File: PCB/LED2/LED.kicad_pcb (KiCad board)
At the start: 2 copper layers, 70 x 70 mm, 29 parts, among them J1 Conn_01x03, J2 USB-C, U1 ESP32-PICO-MINI-02, U2 QR, U3 MD8942, U4 Barcode, U5 CH340X

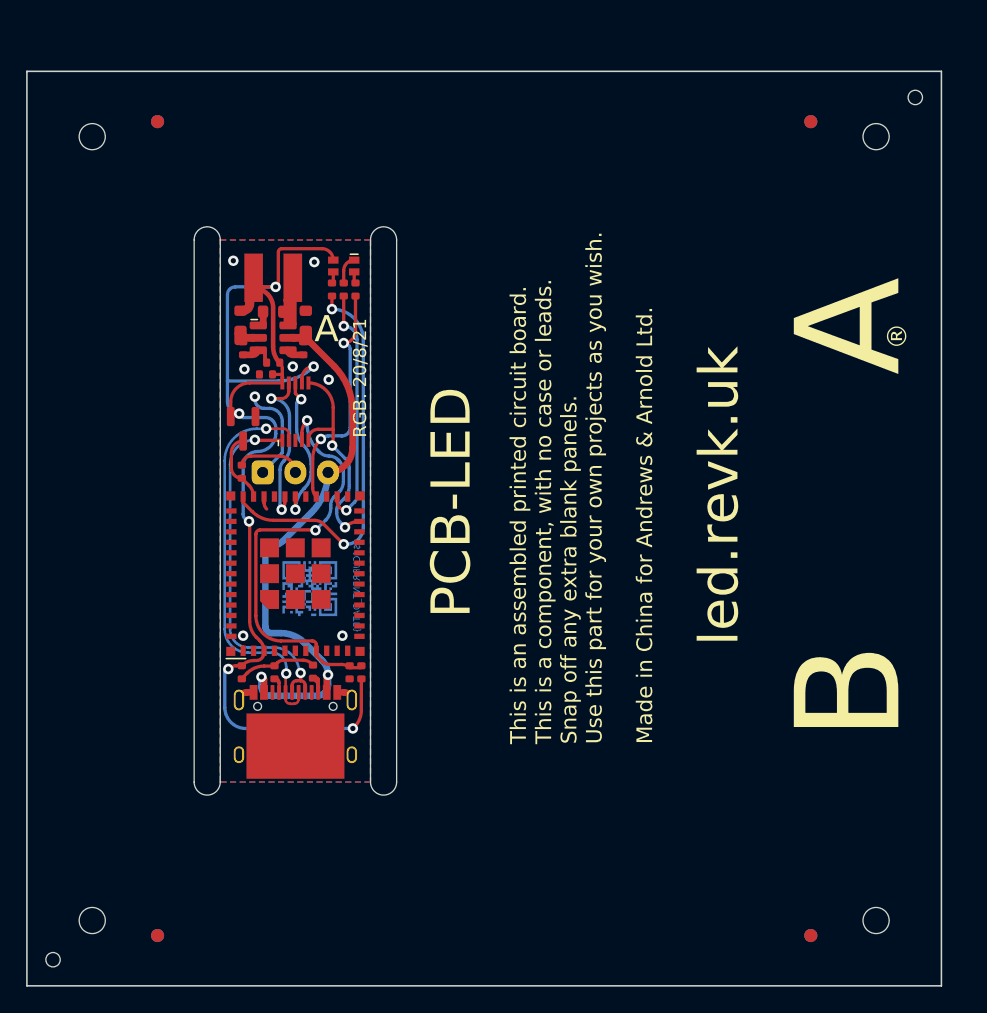
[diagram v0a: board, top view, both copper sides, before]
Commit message: Started tracking
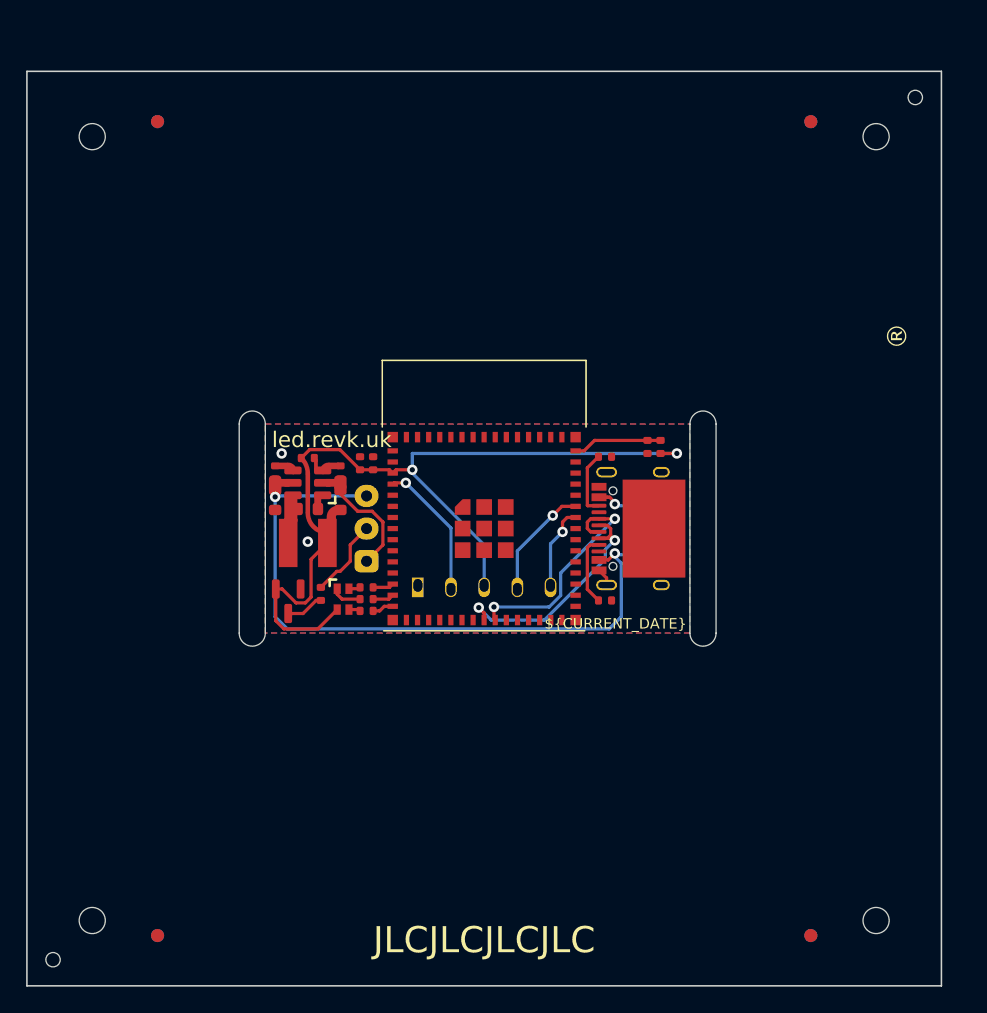
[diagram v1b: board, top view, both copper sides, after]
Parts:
- removed C1: 1uF, RevK:C_0402
- removed C2: 10uF 50V, RevK:C_0603_
- removed C3: 10uF 6.3V, RevK:C_0603_
- removed C4: 100nF, RevK:C_0603_
- removed C5, C6: 100nF, RevK:C_0402
- removed L1: 10uH, RevK:L_4x4_
- removed R1: 10k, RevK:R_0402
- removed R10: 40k2, RevK:R_0402_
- removed R13: 1M, RevK:R_0402_
- removed R9: 124k, RevK:R_0402_
- removed U1: ESP32-PICO-MINI-02, RevK:ESP32-PICO-MINI-02
- removed U2: QR, RevK:QR-LED
- removed U3: MD8942, RevK:SOT-23-6-MD8942
- removed U5: CH340X, RevK:CH340X
- added C10: 10uF 50V, RevK:C_0603_, F.Cu at (84.0, 97.8)
- added C11: 10uF 6.3V, RevK:C_0603_, F.Cu at (89.0, 97.8)
- added C12: 100nF, RevK:C_0603_, F.Cu at (86.5, 98.5)
- added C7: 100nF, RevK:C_0402, F.Cu at (91.5, 95.0)
- added C8: 22uF, RevK:C_0402, F.Cu at (90.5, 95.0)
- added C9: 1uF, RevK:C_0402, F.Cu at (112.5, 93.8)
- added J3: Shelly, RevK:Shelly, B.Cu at (100.0, 104.5)
- added L2: 10uH, RevK:L_4x4_, F.Cu at (86.5, 101.1)
- added R14: 39k2, RevK:R_0402_, F.Cu at (89.0, 95.7)
- added R15: 1M, RevK:R_0402_, F.Cu at (84.0, 95.7)
- added R2: 10K, RevK:R_0402, F.Cu at (113.5, 93.8)
- added R4: 124k, RevK:R_0402_, F.Cu at (86.5, 94.6)
- added U6: ESP32-S3-MINI-1, RevK:ESP32-S3-MINI-1, F.Cu at (100.0, 100.0)
- added U7: MD8942, RevK:SOT-23-6-MD8942, F.Cu at (86.5, 96.5)
- moved U4 31.3 mm to (118.5, 108.4), turned to 180 degrees
- moved J2 29.8 mm to (111.2, 100.0), turned to 90 degrees
- moved R6 27.8 mm to (109.2, 94.5), turned to 180 degrees
- moved R5 25.9 mm to (109.2, 105.5), turned to 0 degrees
- moved D2 25.5 mm to (89.2, 105.4), turned to -90 degrees
- moved R12 24.7 mm to (91.0, 106.3), turned to 0 degrees
- moved R8 23.8 mm to (91.0, 105.4), turned to 0 degrees
- moved R11 22.8 mm to (91.0, 104.5), turned to 0 degrees
- moved V1 14.1 mm to (100.0, 92.0)
- moved D3 13.6 mm to (85.0, 105.6)
- moved V2 11.4 mm to (100.0, 108.0)
- moved R7 11.1 mm to (87.5, 105.0)
- moved J1 6.94 mm to (91.0, 100.0), turned to 90 degrees
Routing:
- net EN: track 33.5 -> 0.00 mm, vias 2 -> 0
- net B: track 30.5 -> 1.64 mm, vias 2 -> 0
- net +3V3: track 83.6 -> 59.5 mm, vias 6 -> 2
- net R: track 18.7 -> 1.62 mm, vias 2 -> 0
- net GPIO0: track 16.7 -> 0.00 mm, vias 2 -> 0
- net G: track 18.1 -> 1.60 mm, vias 2 -> 0
- net DC: track 43.1 -> 58.5 mm, vias 2 -> 3
- net O: track 12.8 -> 0.00 mm, vias 2 -> 0
- net D-: track 30.4 -> 18.6 mm
- net I: track 11.7 -> 0.00 mm, vias 2 -> 0
- net Net-(J3-0): track 0.00 -> 10.6 mm, vias 0 -> 1
- net D+: track 27.9 -> 17.8 mm
- net Net-(J3-Rx): track 0.00 -> 8.81 mm, vias 0 -> 1
- net GND: track 17.4 -> 9.35 mm, vias 8 -> 2
- net Net-(U6-EN): track 0.00 -> 6.83 mm
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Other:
- board text added: "5060634238090"
- board text added: "Made in China for Andresw&Arnold Ltd"
- board text removed: "${TITLE}"
- board text removed: "22"
- board text removed: "RGB: 20/8/21"
- board text removed: "This is an assembled printed circuit board. This is a component, with no case or leads. Snap off any extra blank panels. Use this part for your own projects as you wish. Made in China for Andrews & Arnold Ltd."

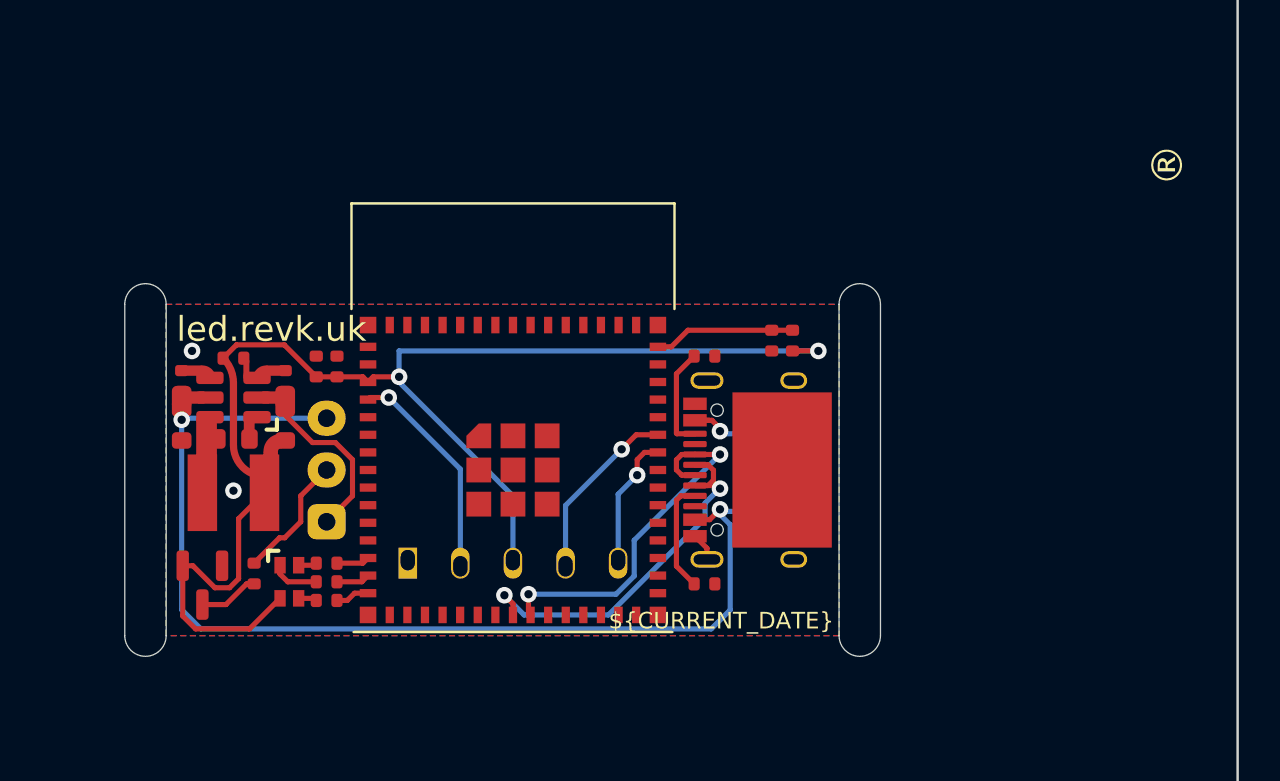
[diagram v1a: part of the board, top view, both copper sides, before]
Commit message: Tracked
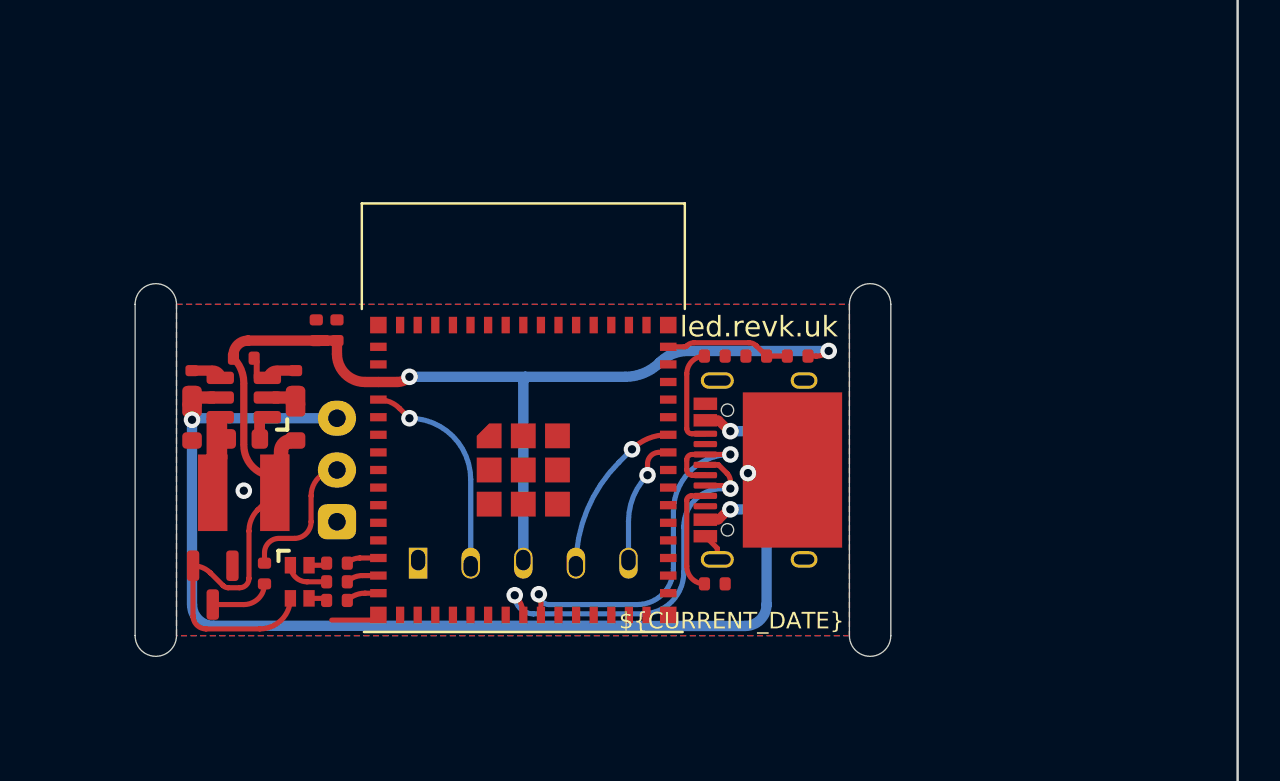
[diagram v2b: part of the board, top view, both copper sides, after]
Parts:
- moved C7 1.75 mm to (91.5, 93.2)
- moved C8 1.75 mm to (90.5, 93.2)
- moved C9 1.06 mm to (111.8, 94.5), turned to 180 degrees
- moved R2 0.79 mm to (113.8, 94.5), turned to 180 degrees
- moved C10 0.50 mm to (84.5, 97.8)
- moved C11 0.50 mm to (89.5, 97.8)
- moved C12 0.50 mm to (87.0, 98.5)
- moved D2 0.50 mm to (89.7, 105.4)
- moved D3 0.50 mm to (85.5, 105.6)
- moved J1 0.50 mm to (91.5, 100.0)
- moved J2 0.50 mm to (111.8, 100.0)
- moved J3 0.50 mm to (100.5, 104.5)
- moved L2 0.50 mm to (87.0, 101.1)
- moved R11 0.50 mm to (91.5, 104.5)
- moved R12 0.50 mm to (91.5, 106.3)
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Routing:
- net GND: track 9.35 -> 3.61 mm
- net DC: track 58.5 -> 61.0 mm
- net +3V3: track 59.5 -> 57.6 mm
- net D+: track 17.8 -> 19.4 mm
- net D-: track 18.6 -> 19.5 mm
- net Net-(U6-EN): track 6.83 -> 6.04 mm
- net Net-(J1-Pin_2): track 6.10 -> 6.71 mm
- net Net-(J3-Rx): track 8.81 -> 8.30 mm
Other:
- board text removed: "®"

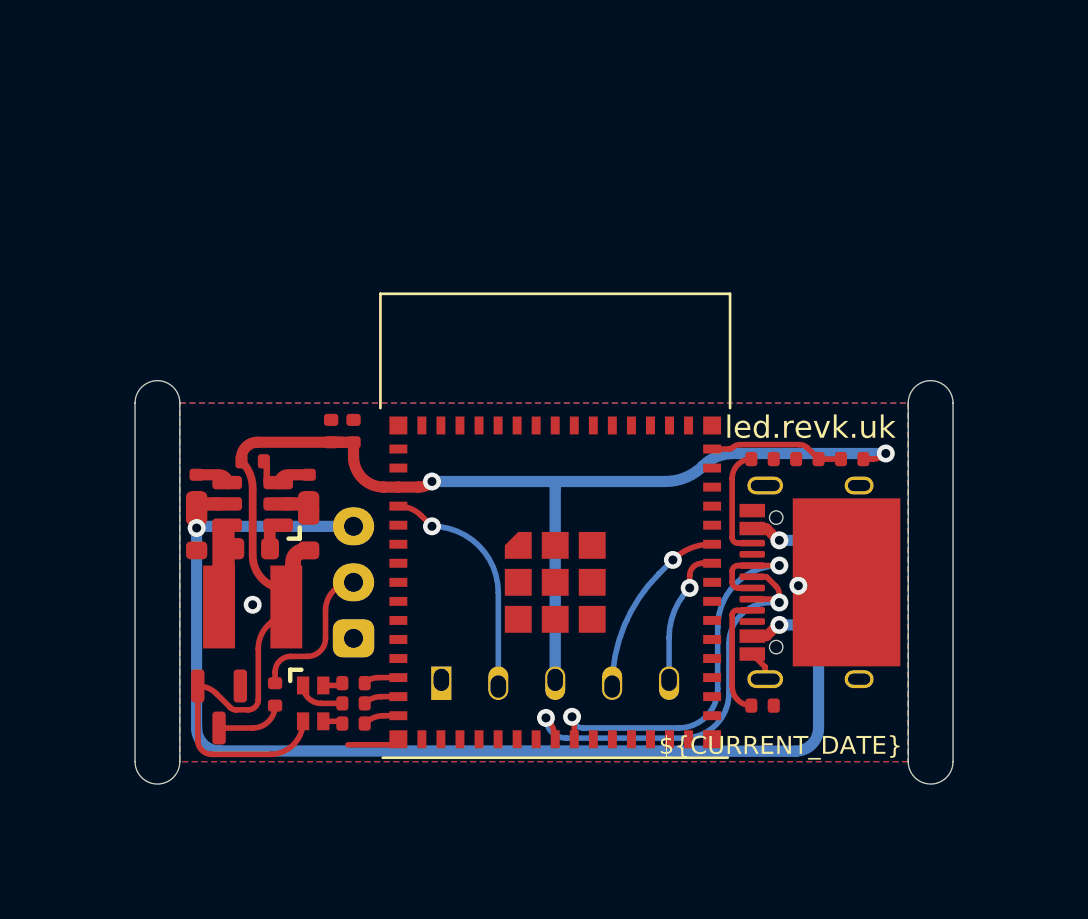
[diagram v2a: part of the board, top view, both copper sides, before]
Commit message: New S3
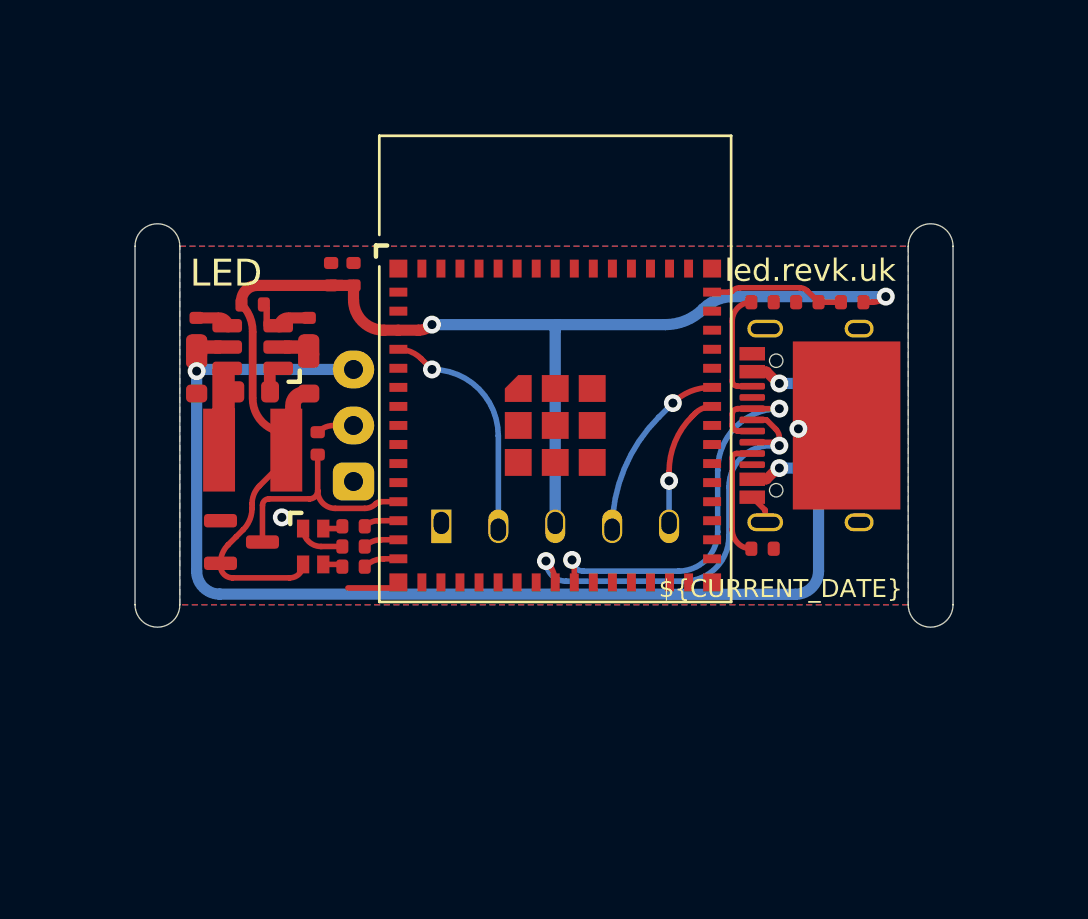
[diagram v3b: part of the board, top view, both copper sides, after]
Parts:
- moved R7 11.4 mm to (89.9, 93.8)
- moved D3 7.43 mm to (86.5, 98.2), turned to 0 degrees
- moved C10 7.00 mm to (84.5, 90.8)
- moved C11 7.00 mm to (89.5, 90.8)
- moved C12 7.00 mm to (87.0, 91.5)
- moved C7 7.00 mm to (91.5, 86.2)
- moved C8 7.00 mm to (90.5, 86.2)
- moved C9 7.00 mm to (111.8, 87.5)
- moved D2 7.00 mm to (89.7, 98.4)
- moved J1 7.00 mm to (91.5, 93.0)
- moved J2 7.00 mm to (111.8, 93.0)
- moved J3 7.00 mm to (100.5, 97.5)
- moved L2 7.00 mm to (87.0, 94.1)
- moved R11 7.00 mm to (91.5, 97.5)
- moved R12 7.00 mm to (91.5, 99.3)
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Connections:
- U6 pad 12: unconnected-(U6-GPIO8-Pad12) -> LED
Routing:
- net LED: track 3.03 -> 10.2 mm
- net +3V3: track 57.6 -> 51.9 mm
- net Net-(J1-Pin_2): track 6.71 -> 1.68 mm
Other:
- board text added: "Made in China for Andresw & Arnold Ltd"
- board text removed: "Made in China for Andresw&Arnold Ltd"
